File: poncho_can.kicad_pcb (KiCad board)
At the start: 2 copper layers, 85.7 x 79.6 mm, 40 parts, among them J10 GS2, J101 DB9_Male_MountingHoles, J102 DB9_Male_MountingHoles, J103 GS2, J104 GS2, J105 GS2, J106 GS2, J7 GS2, J8 GS2, J9 GS2, U101 TJA1051T, U102 TJA1051T

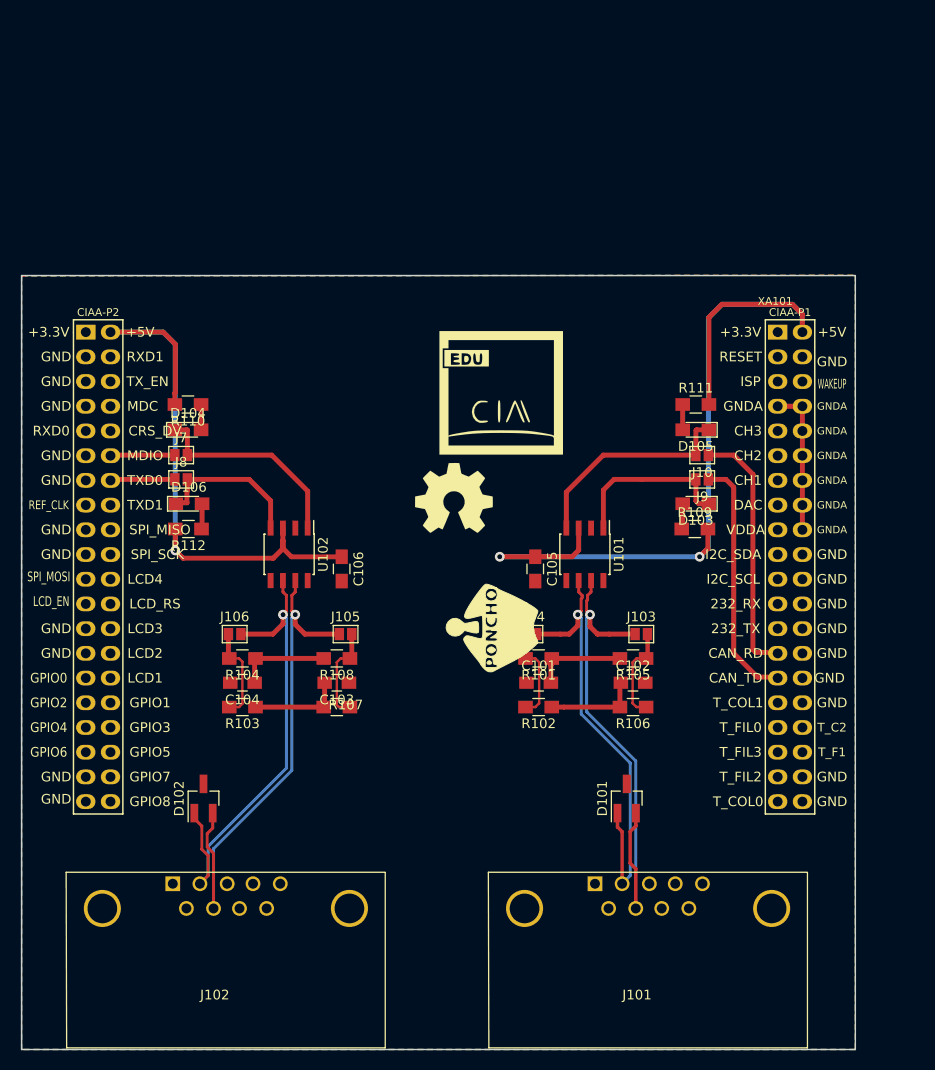
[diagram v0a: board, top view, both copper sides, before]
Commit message: Fin de esquematico y agrego los gerbers
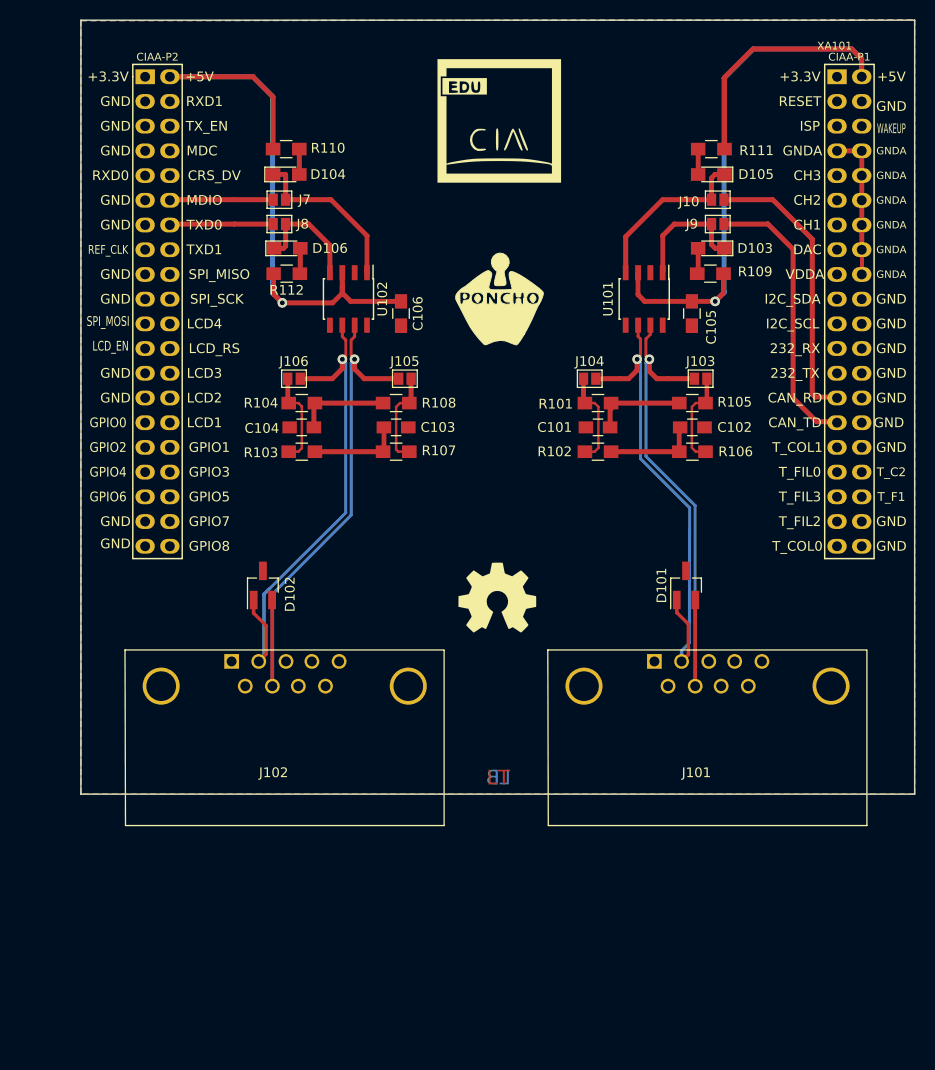
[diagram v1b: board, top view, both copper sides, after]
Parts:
- moved G*** 33.8 mm to (108.8, 83.1), turned to 0 degrees
- moved C105 30.8 mm to (128.6, 84.5)
- moved D104 28.1 mm to (86.9, 70.2)
- moved J7 28.1 mm to (86.2, 72.8)
- moved J8 28.1 mm to (86.2, 75.3)
- moved R110 28.1 mm to (86.9, 67.7)
- moved R112 28.1 mm to (87.0, 80.5)
- moved D106 28.1 mm to (87.0, 77.8)
- moved G*** 28.0 mm to (108.8, 64.8)
- moved C101 26.9 mm to (119.0, 96.2)
- moved C102 26.9 mm to (128.7, 96.2)
- moved C103 26.9 mm to (98.2, 96.2)
- moved C106 26.9 mm to (98.7, 84.5)
- moved J106 26.9 mm to (87.7, 91.2)
- moved R101 26.9 mm to (119.0, 93.8)
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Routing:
- net GNDA: track 15.2 -> 38.1 mm
- net +5V: track 93.2 -> 82.0 mm, vias 2 -> 1
- net Net-(D105-Pad1): track 22.5 -> 17.8 mm
- net Net-(D103-Pad1): track 17.3 -> 12.9 mm
- net Net-(D106-Pad1): track 15.9 -> 11.8 mm
- net Net-(D104-Pad1): track 21.6 -> 17.5 mm
- net +5VP: track 65.1 -> 69.1 mm
- net Net-(J7-Pad1): track 6.64 -> 10.6 mm
- net Net-(J8-Pad1): track 6.66 -> 10.7 mm
- net Net-(J9-Pad1): track 25.3 -> 28.7 mm
- net Net-(J10-Pad1): track 25.8 -> 29.1 mm
- net /CAN1-: track 47.3 -> 50.2 mm
- net /CAN2-: track 49.2 -> 52.0 mm
- net Net-(J104-Pad1): track 7.34 -> 9.89 mm
- net /CAN2+: track 53.7 -> 55.7 mm
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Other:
- net class Default: clearance 0.254 -> 0.1524
- rule trace_clearance: 0.254 -> 0.1524
- board text added: "LB"
- board text added: "LT"
- board text added: "PONCHO CAN http://www.proyecto-ciaa.com.ar/"
- board text removed: "Borrar (Footprint MP1) la Plantilla-EDU-CIAA al finalizar el posicionamiento y definido el borde de PCB."
- board text removed: "PONCHO BASICO http://www.proyecto-ciaa.com.ar/"
- board text removed: "Se sugiere colocar Nombre de Poncho y autor en cobre, serigrafía y rótulo."
